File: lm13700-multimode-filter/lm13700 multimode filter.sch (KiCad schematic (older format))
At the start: 49 parts, among them J1 Power In, J2 Audio In, J3 CV-in, J4 High Pass, J5 Band Pass, J6 Low pass, Q1 2N3906, Q2 2N3906, U1 TL074, U2 TL072, U3 LM13700

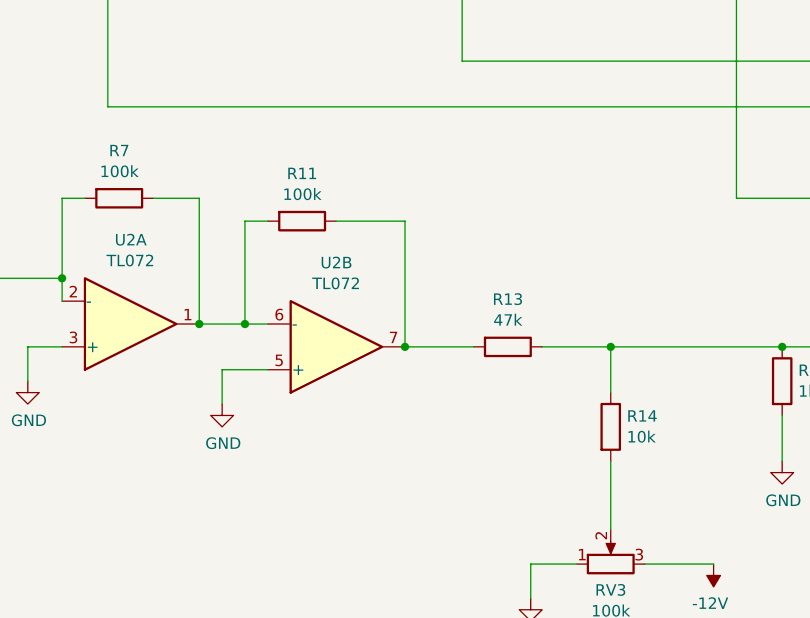
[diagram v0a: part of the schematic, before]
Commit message: add: panels
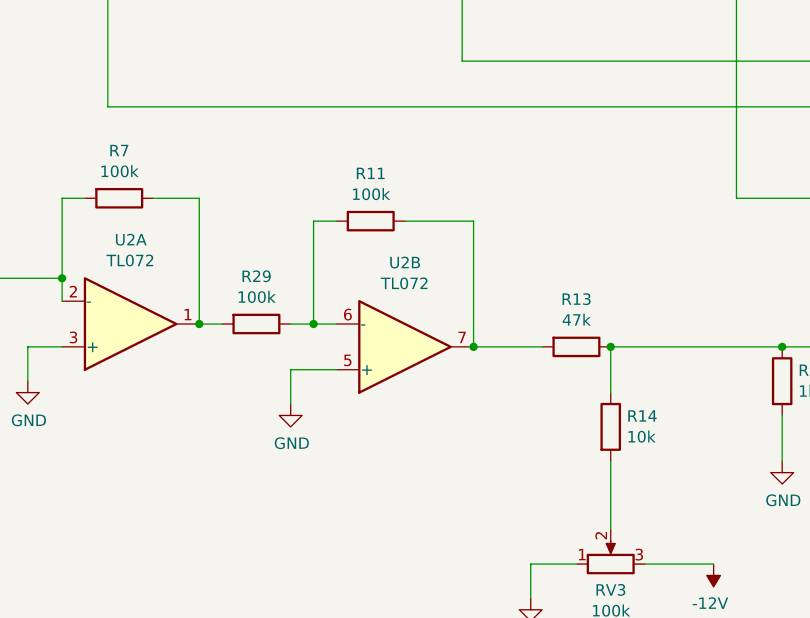
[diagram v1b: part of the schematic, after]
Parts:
- added R29: 100k, Resistor_THT:R_Axial_DIN0207_L6.3mm_D2.5mm_P7.62mm_Horizontal, symbol Device:R
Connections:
- net at R7.1, U2.1: now also R29.2; no longer R11.2, U2.6 (-)
- new net: R11.2, R29.1, U2.6 (-)
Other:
- moved on the sheet: R11, R13, U2B
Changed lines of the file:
@@
 L power:GND #PWR014
 U 1 1 602599EB
-P 3550 4800
-F 0 "#PWR014" H 3550 4550 50  0001 C CNN
-F 1 "GND" H 3555 4627 50  0000 C CNN
-F 2 "" H 3550 4800 50  0001 C CNN
-F 3 "" H 3550 4800 50  0001 C CNN
-	1    3550 4800
-	1    0    0    -1
-$EndComp
-Wire Wire Line
-	3750 4650 3550 4650
-Wire Wire Line
-	3550 4650 3550 4800
+P 3850 4800
+F 0 "#PWR014" H 3850 4550 50  0001 C CNN
+F 1 "GND" H 3855 4627 50  0000 C CNN
+F 2 "" H 3850 4800 50  0001 C CNN
+F 3 "" H 3850 4800 50  0001 C CNN
+	1    3850 4800
+	1    0    0    -1
+$EndComp
+Wire Wire Line
+	4050 4650 3850 4650
+Wire Wire Line
+	3850 4650 3850 4800
 $Comp
 L Device:R R11
 U 1 1 6025C2E8
-P 3900 4000
-F 0 "R11" V 3693 4000 50  0000 C CNN
-F 1 "100k" V 3784 4000 50  0000 C CNN
-F 2 "Resistor_THT:R_Axial_DIN0207_L6.3mm_D2.5mm_P7.62mm_Horizontal" V 3830 4000 50  0001 C CNN
-F 3 "~" H 3900 4000 50  0001 C CNN
-	1    3900 4000
+P 4200 4000
+F 0 "R11" V 3993 4000 50  0000 C CNN
+F 1 "100k" V 4084 4000 50  0000 C CNN
+F 2 "Resistor_THT:R_Axial_DIN0207_L6.3mm_D2.5mm_P7.62mm_Horizontal" V 4130 4000 50  0001 C CNN
+F 3 "~" H 4200 4000 50  0001 C CNN
+	1    4200 4000
 	0    1    1    0
 $EndComp
 Wire Wire Line
-	3450 4450 3650 4450
-Wire Wire Line
-	3750 4000 3650 4000
-Wire Wire Line
-	3650 4000 3650 4450
-Connection ~ 3650 4450
-Wire Wire Line
-	3650 4450 3750 4450
-Wire Wire Line
-	4050 4000 4350 4000
-Wire Wire Line
-	4350 4000 4350 4550
+	4050 4000 3950 4000
+Wire Wire Line
+	3950 4000 3950 4450
+Wire Wire Line
+	3950 4450 4050 4450
+Wire Wire Line
+	4350 4000 4650 4000
+Wire Wire Line
+	4650 4000 4650 4550
 $Comp
 L Device:R R13
 U 1 1 602644D6
-P 4800 4550
-F 0 "R13" V 4593 4550 50  0000 C CNN
-F 1 "47k" V 4684 4550 50  0000 C CNN
-F 2 "Resistor_THT:R_Axial_DIN0207_L6.3mm_D2.5mm_P7.62mm_Horizontal" V 4730 4550 50  0001 C CNN
-F 3 "~" H 4800 4550 50  0001 C CNN
-	1    4800 4550
+P 5100 4550
+F 0 "R13" V 4893 4550 50  0000 C CNN
+F 1 "47k" V 4984 4550 50  0000 C CNN
+F 2 "Resistor_THT:R_Axial_DIN0207_L6.3mm_D2.5mm_P7.62mm_Horizontal" V 5030 4550 50  0001 C CNN
+F 3 "~" H 5100 4550 50  0001 C CNN
+	1    5100 4550
 	0    1    1    0
 $EndComp
 Wire Wire Line
-	4350 4550 4650 4550
+	4650 4550 4950 4550
 $Comp
 L Device:R R14
@@
 Wire Wire Line
 	5700 5500 5400 5500
-Wire Wire Line
-	4950 4550 5250 4550
 $Comp
 L Device:R R16
@@
 Wire Wire Line
 	5250 4550 6000 4550
-Connection ~ 5250 4550
 $Comp
 L power:GND #PWR023
@@
 	1    0    0    1
 $EndComp
-Connection ~ 3450 4450
 $Comp
 L Amplifier_Operational:TL072 U2
 U 2 1 602EB081
-P 4050 4550
-F 0 "U2" H 4050 4183 50  0000 C CNN
-F 1 "TL072" H 4050 4274 50  0000 C CNN
-F 2 "Package_DIP:DIP-8_W7.62mm_Socket" H 4050 4550 50  0001 C CNN
-F 3 "http://www.ti.com/lit/ds/symlink/tl071.pdf" H 4050 4550 50  0001 C CNN
-	2    4050 4550
+P 4350 4550
+F 0 "U2" H 4350 4183 50  0000 C CNN
+F 1 "TL072" H 4350 4274 50  0000 C CNN
+F 2 "Package_DIP:DIP-8_W7.62mm_Socket" H 4350 4550 50  0001 C CNN
+F 3 "http://www.ti.com/lit/ds/symlink/tl071.pdf" H 4350 4550 50  0001 C CNN
+	2    4350 4550
 	1    0    0    1
 $EndComp
-Connection ~ 4350 4550
+Connection ~ 4650 4550
 $Comp
 L Amplifier_Operational:TL072 U2
@@
 	-1   0    0    1
 $EndComp
+Connection ~ 5250 4550
+$Comp
+L Device:R R29
+U 1 1 617FB1CE
+P 3700 4450
+F 0 "R29" V 3493 4450 50  0000 C CNN
+F 1 "100k" V 3584 4450 50  0000 C CNN
+F 2 "Resistor_THT:R_Axial_DIN0207_L6.3mm_D2.5mm_P7.62mm_Horizontal" V 3630 4450 50  0001 C CNN
+F 3 "~" H 3700 4450 50  0001 C CNN
+	1    3700 4450
+	0    1    1    0
+$EndComp
+Wire Wire Line
+	3550 4450 3450 4450
+Connection ~ 3450 4450
+Wire Wire Line
+	3850 4450 3950 4450
+Connection ~ 3950 4450
 $EndSCHEMATC
